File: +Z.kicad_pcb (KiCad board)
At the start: 4 copper layers, 98 x 98 mm, 225 parts, among them J1 522711069, Q1 MBT2222ADW1T1, Q10 NX3008NBKS, Q11 MBT2222ADW1T1, Q12 NX3008NBKS, Q13 MBT2222ADW1T1, Q14 NX3008NBKS, Q15 MBT2222ADW1T1, Q16 NX3008NBKS, Q17 SIRA99DP-T1-GE3, Q18 MBT2222ADW1T1, Q19 NX3008NBKS, Q2 NX3008NBKS, Q20 MBT2222ADW1T1, Q21 NX3008NBKS, Q22 IRLML2803, Q23 SIRA99DP-T1-GE3, Q24 MBT2222ADW1T1, Q25 NX3008NBKS, Q26 MBT2222ADW1T1, Q27 NX3008NBKS, Q3 MBT2222ADW1T1, Q4 NX3008NBKS, Q5 MBT2222ADW1T1, Q6 NX3008NBKS, Q7 MBT2222ADW1T1, Q8 NX3008NBKS, Q9 MBT2222ADW1T1, U1 SunSensor, U10 LTC4316IDD, U2 SunSensor, U3 SunSensor, U4 SunSensor, U5 ADM1176-1ARMZ-R7, U6 LTC3130IUDC, U7 LTC4412xS6, U8 DRV8235RTER, U9 D5V0P4UR6SO

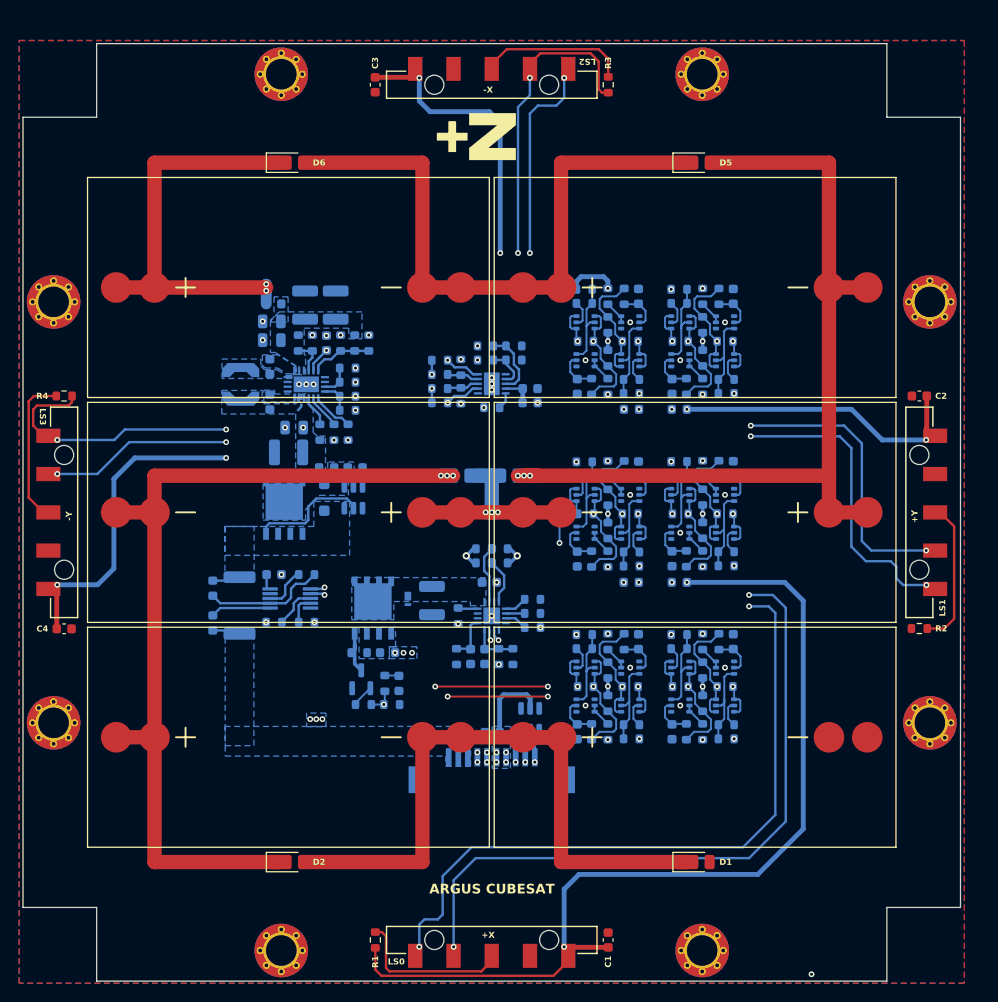
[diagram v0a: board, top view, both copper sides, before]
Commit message: V4 Updates
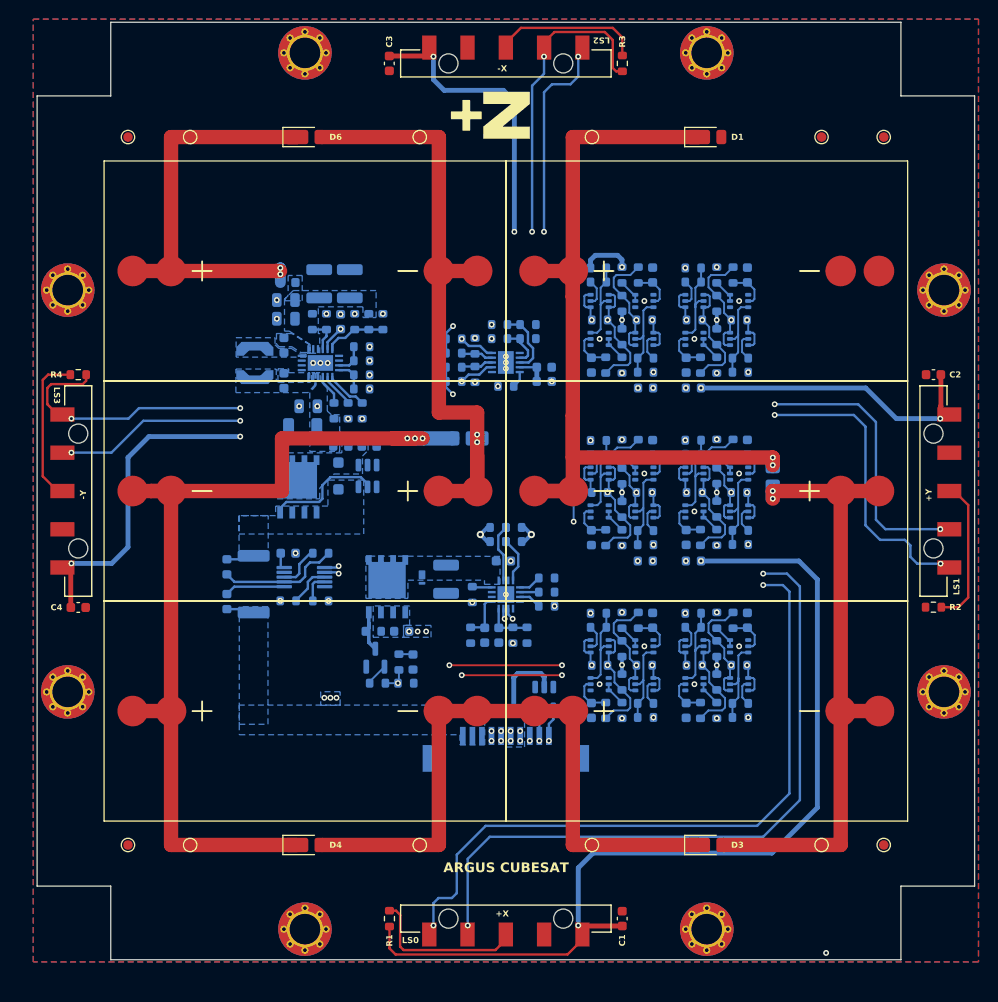
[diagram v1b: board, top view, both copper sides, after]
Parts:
- added H10: MountingHole_Pad, TestPoint:TestPoint_Pad_D1.0mm, F.Cu at (161.3, 58.0)
- added H11: MountingHole_Pad, TestPoint:TestPoint_Pad_D1.0mm, F.Cu at (185.3, 132.0)
- added H12: MountingHole_Pad, TestPoint:TestPoint_Pad_D1.0mm, F.Cu at (143.3, 132.0)
- added H13: MountingHole_Pad, TestPoint:TestPoint_Pad_D1.0mm, F.Cu at (119.3, 132.0)
- added H14: MountingHole_Pad, TestPoint:TestPoint_Pad_D1.0mm, F.Cu at (143.3, 58.0)
- added H15: MountingHole_Pad, TestPoint:TestPoint_Pad_D1.0mm, F.Cu at (119.3, 58.0)
- added H16: MountingHole_Pad, TestPoint:TestPoint_Pad_D1.0mm, F.Cu at (161.3, 132.0)
- added H17: MountingHole_Pad, TestPoint:TestPoint_Pad_D1.0mm, F.Cu at (191.8, 58.0)
- added H18: MountingHole_Pad, TestPoint:TestPoint_Pad_D1.0mm, F.Cu at (112.8, 58.0)
- added H19: MountingHole_Pad, TestPoint:TestPoint_Pad_D1.0mm, F.Cu at (191.8, 132.0)
- added H20: MountingHole_Pad, TestPoint:TestPoint_Pad_D1.0mm, F.Cu at (112.8, 132.0)
- added H9: MountingHole_Pad, TestPoint:TestPoint_Pad_D1.0mm, F.Cu at (185.3, 58.0)
- D2, D5: moved to B.Cu
- D3, D4: moved to F.Cu
- moved D1 75.8 mm to (173.3, 58.0)
- moved D2 64.3 mm to (180.2, 94.2), turned to 90 degrees
- moved SC2 50.7 mm to (173.3, 95.0), turned to 0 degrees
- moved SC1 48.8 mm to (173.3, 72.0)
- moved SC3 48.4 mm to (173.3, 118.0), turned to 180 degrees
- moved SC5 46.0 mm to (131.3, 95.0), turned to 0 degrees
- moved D3 46.0 mm to (173.3, 132.0), turned to 0 degrees
- moved SC4 45.8 mm to (131.3, 118.0), turned to 180 degrees
- moved D4 44.5 mm to (131.3, 132.0), turned to 0 degrees
- moved D5 37.3 mm to (148.4, 89.5), turned to 180 degrees
- moved H1 3.55 mm to (198.1, 116.0)
- moved H4 3.55 mm to (106.5, 116.0)
- moved H6 3.33 mm to (131.3, 140.8)
- moved H7 3.33 mm to (131.3, 49.2)
- moved D6 3.19 mm to (131.3, 58.0)
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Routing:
- net /Coil Driver/coil: track 16395.6 -> 16494.7 mm
- net Net-(D3-K): track 22.0 -> 66.8 mm, vias 3 -> 0
- net Net-(D2-K): track 93.7 -> 64.7 mm, vias 3 -> 2
- net Net-(D1-K): track 70.0 -> 91.8 mm, vias 0 -> 2
- net SCL: track 92.7 -> 104.9 mm
- net Net-(D4-K): track 90.7 -> 100.5 mm
- net SDA: track 81.5 -> 91.0 mm
- net /Sun Pyramid/LS3_3V3: track 110.9 -> 104.3 mm
- net /Sun Pyramid/LS3_SCL: track 77.7 -> 73.2 mm
- net /Sun Pyramid/LS3_SDA: track 88.8 -> 84.5 mm
- net SCL_LS: track 119.5 -> 121.9 mm
- net SDA_LS: track 71.0 -> 69.5 mm
- net Net-(D5-K): track 65.9 -> 64.9 mm, vias 0 -> 2
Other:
- board text added: "ARGUS Cubesat Carnegie Mellon University +Z Solar Panel v4.0"
- board text removed: "ARGUS Cubesat Carnegie Mellon University +Z Solar Panel v3.1"

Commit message: Coil direction comment clarification
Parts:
- R55: value 0R -> 150k
